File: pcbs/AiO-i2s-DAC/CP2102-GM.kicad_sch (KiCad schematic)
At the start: 12 parts, among them U4 CP2102-GM

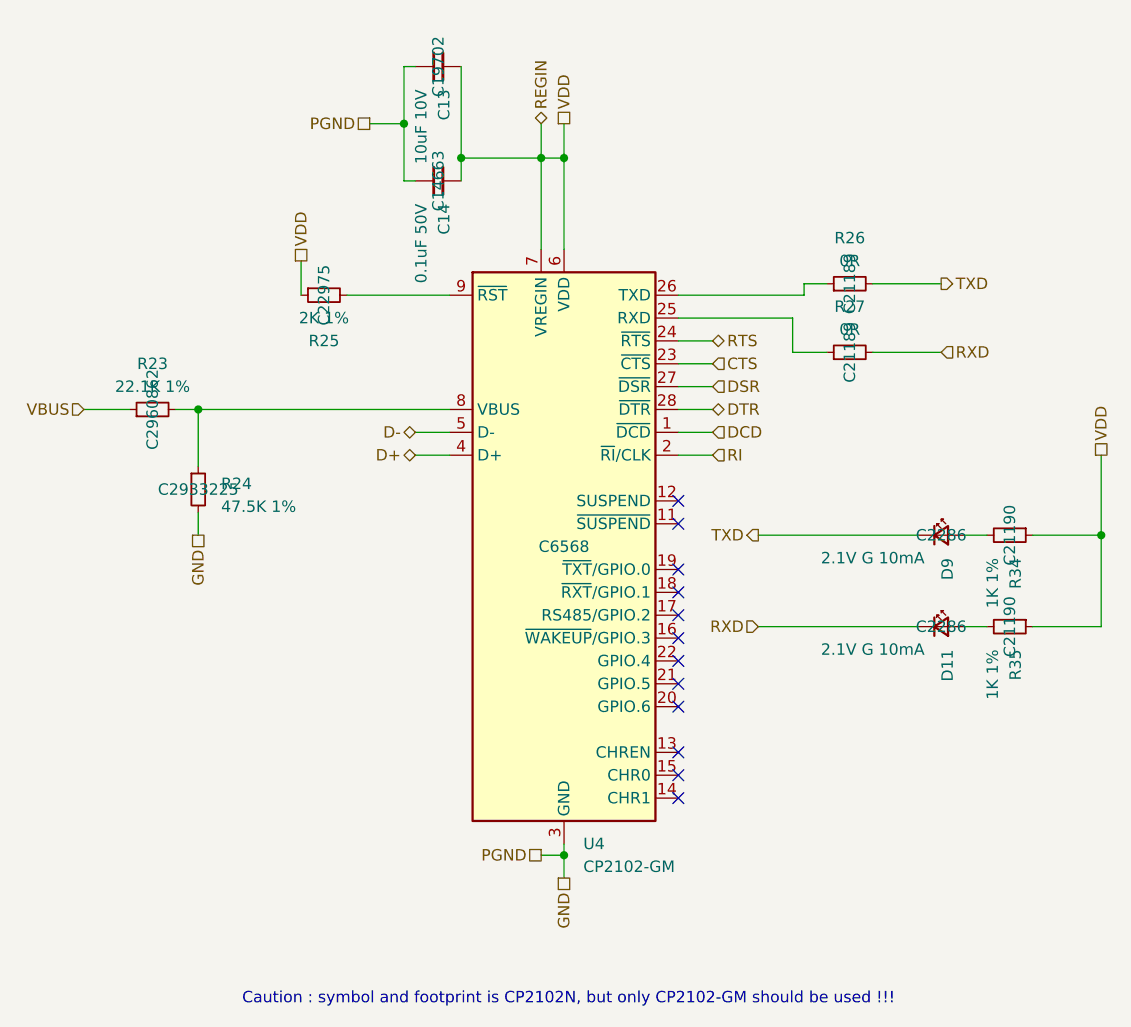
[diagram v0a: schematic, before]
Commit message: LCSC BOM Preparation
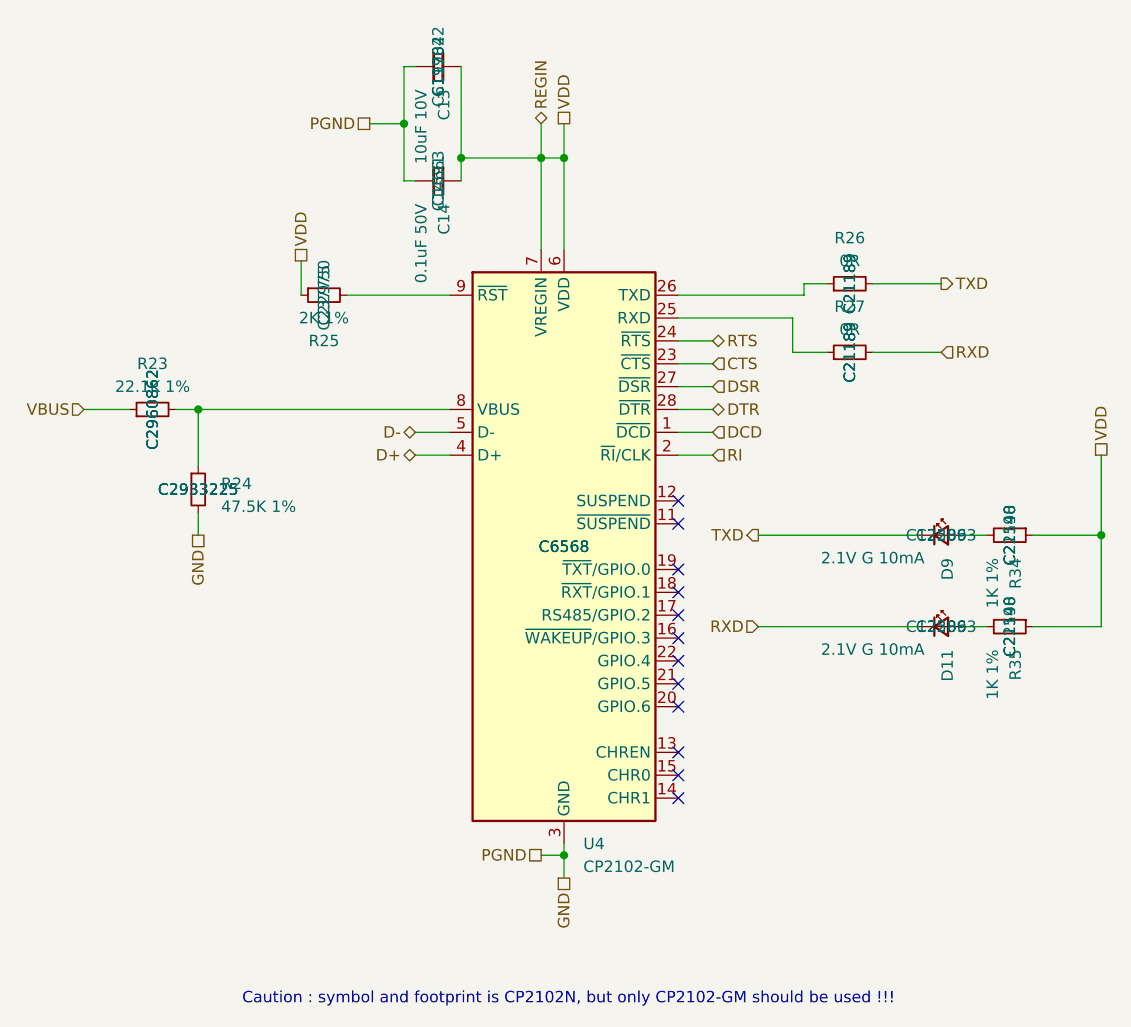
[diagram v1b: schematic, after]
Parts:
- C13: LCSC alt (none) -> C6119842
- C14: LCSC alt (none) -> C1591
- D11, D9: LCSC alt (none) -> C125093
- R23: LCSC alt (none) -> C2960862
- R24: LCSC alt (none) -> C2933225
- R25: LCSC alt (none) -> C237750
- R26, R27: LCSC alt (none) -> C21189
- R34, R35: LCSC alt (none) -> C22548
- U4: LCSC alt (none) -> C6568
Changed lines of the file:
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@@
+			)
+		)
+		(property "LCSC alt" "C22548"
+			(at 203.2 100.33 0)
+			(effects
+				(font
+					(size 1.27 1.27)
+				)
 			)
 		)
@@
 			)
 		)
+		(property "LCSC alt" "C1591"
+			(at 139.7 60.96 0)
+			(effects
+				(font
+					(size 1.27 1.27)
+				)
+			)
+		)
 		(pin "1"
 		)
@@
 			)
 		)
+		(property "LCSC alt" "C125093"
+			(at 195.58 110.49 0)
+			(effects
+				(font
+					(size 1.27 1.27)
+				)
+			)
+		)
 		(pin "1"
 		)
@@
 		)
 		(property "LCSC" "C2286"
+			(at 195.58 100.33 0)
+			(effects
+				(font
+					(size 1.27 1.27)
+				)
+			)
+		)
+		(property "LCSC alt" "C125093"
 			(at 195.58 100.33 0)
 			(effects
@@
 			)
 		)
+		(property "LCSC alt" "C21189"
+			(at 185.42 80.01 0)
+			(effects
+				(font
+					(size 1.27 1.27)
+				)
+			)
+		)
 		(pin "1"
 		)
@@
 			)
 		)
+		(property "LCSC alt" "C6119842"
+			(at 139.7 48.26 0)
+			(effects
+				(font
+					(size 1.27 1.27)
+				)
+			)
+		)
 		(pin "1"
 		)
@@
 			)
 		)
+		(property "LCSC alt" "C2960862"
+			(at 107.95 86.36 0)
+			(effects
+				(font
+					(size 1.27 1.27)
+				)
+			)
+		)
 		(pin "1"
 		)
@@
 			)
 		)
+		(property "LCSC alt" "C22548"
+			(at 203.2 110.49 0)
+			(effects
+				(font
+					(size 1.27 1.27)
+				)
+			)
+		)
 		(pin "1"
 		)
@@
 			)
 		)
+		(property "LCSC alt" "C21189"
+			(at 185.42 72.39 0)
+			(effects
+				(font
+					(size 1.27 1.27)
+				)
+			)
+		)
 		(pin "1"
 		)
@@
 			)
 		)
+		(property "LCSC alt" "C237750"
+			(at 127 73.66 0)
+			(effects
+				(font
+					(size 1.27 1.27)
+				)
+			)
+		)
 		(pin "1"
 		)
@@
 			)
 		)
+		(property "LCSC alt" "C2933225"
+			(at 113.03 95.25 0)
+			(effects
+				(font
+					(size 1.27 1.27)
+				)
+			)
+		)
 		(pin "1"
 		)
@@
 			(at 153.67 101.6 0)
 			(effects
+				(font
+					(size 1.27 1.27)
+				)
+			)
+		)
+		(property "LCSC alt" "C6568"
+			(at 153.67 101.6 0)
+			(effects

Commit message: Build prep
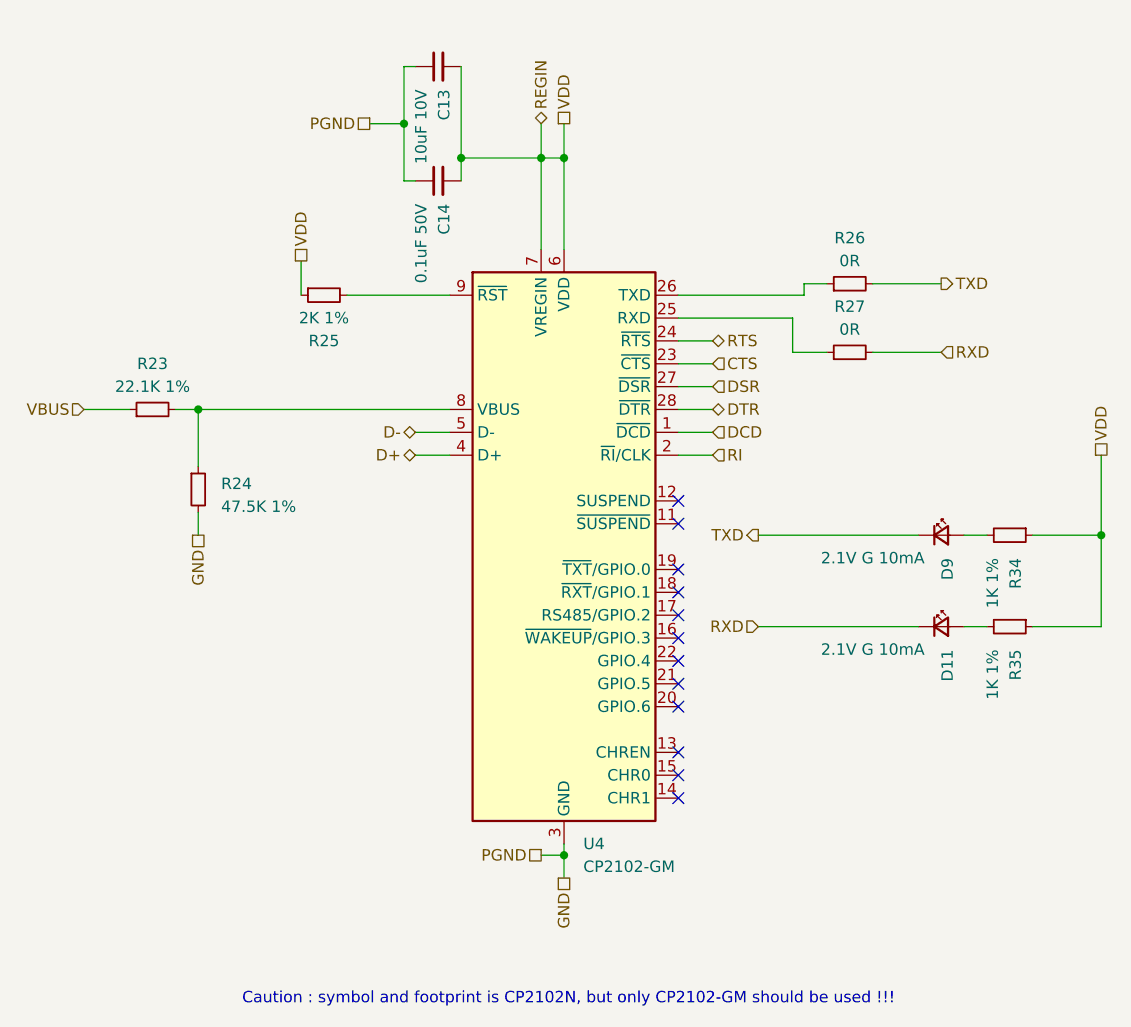
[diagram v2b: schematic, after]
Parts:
- R23: LCSC C2960862 -> C6397988
- R24: LCSC C2933225 -> C403243
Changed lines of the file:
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@@
 					(size 1.27 1.27)
 				)
+				(hide yes)
 			)
 		)
@@
 					(size 1.27 1.27)
 				)
+				(hide yes)
 			)
 		)
@@
 					(size 1.27 1.27)
 				)
+				(hide yes)
 			)
 		)
@@
 					(size 1.27 1.27)
 				)
+				(hide yes)
 			)
 		)
@@
 					(size 1.27 1.27)
 				)
+				(hide yes)
 			)
 		)
@@
 					(size 1.27 1.27)
 				)
+				(hide yes)
 			)
 		)
@@
 					(size 1.27 1.27)
 				)
+				(hide yes)
 			)
 		)
@@
 					(size 1.27 1.27)
 				)
+				(hide yes)
 			)
 		)
@@
 					(size 1.27 1.27)
 				)
+				(hide yes)
 			)
 		)
@@
 					(size 1.27 1.27)
 				)
+				(hide yes)
 			)
 		)
@@
 					(size 1.27 1.27)
 				)
+				(hide yes)
 			)
 		)
@@
 					(size 1.27 1.27)
 				)
+				(hide yes)
 			)
 		)
@@
 			)
 		)
-		(property "LCSC" "C2960862"
+		(property "LCSC" "C6397988"
 			(at 107.95 86.36 0)
 			(effects
@@
 					(size 1.27 1.27)
 				)
+				(hide yes)
 			)
 		)
@@
 					(size 1.27 1.27)
 				)
+				(hide yes)
 			)
 		)
@@
 					(size 1.27 1.27)
 				)
+				(hide yes)
 			)
 		)
@@
 					(size 1.27 1.27)
 				)
+				(hide yes)
 			)
 		)
@@
 					(size 1.27 1.27)
 				)
+				(hide yes)
 			)
 		)
@@
 					(size 1.27 1.27)
 				)
+				(hide yes)
 			)
 		)
@@
 					(size 1.27 1.27)
 				)
+				(hide yes)
 			)
 		)
@@
 					(size 1.27 1.27)
 				)
+				(hide yes)
 			)
 		)
@@
 			)
 		)
-		(property "LCSC" "C2933225"
+		(property "LCSC" "C403243"
 			(at 113.03 95.25 0)
 			(effects
@@
 					(size 1.27 1.27)
 				)
+				(hide yes)
 			)
 		)
@@
 					(size 1.27 1.27)
 				)
+				(hide yes)
 			)
 		)
@@
 					(size 1.27 1.27)
 				)
+				(hide yes)
 			)
 		)
@@
 					(size 1.27 1.27)
 				)
-			)
-		)
+				(hide yes)
+			)
+		)
